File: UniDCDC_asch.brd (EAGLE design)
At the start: 35.2 x 35.9 mm, 13 parts

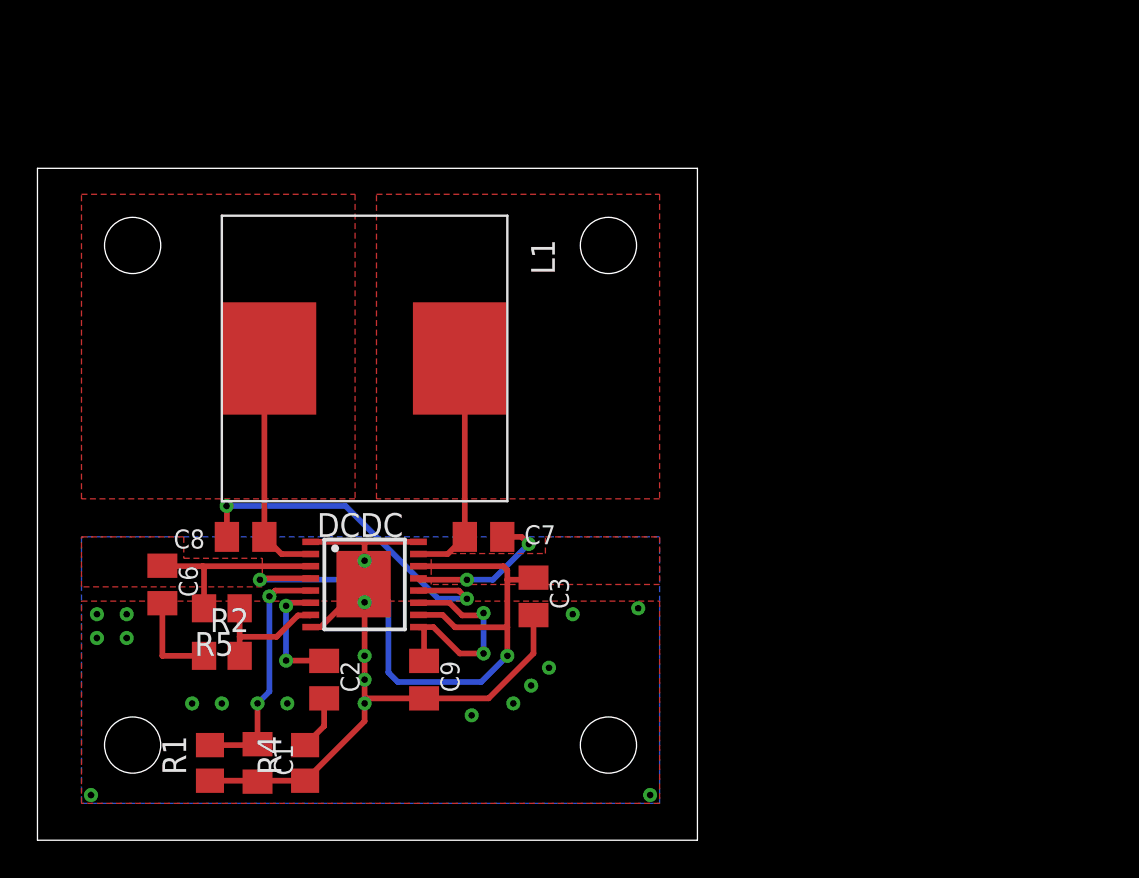
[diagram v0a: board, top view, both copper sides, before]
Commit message: Manufacturing version
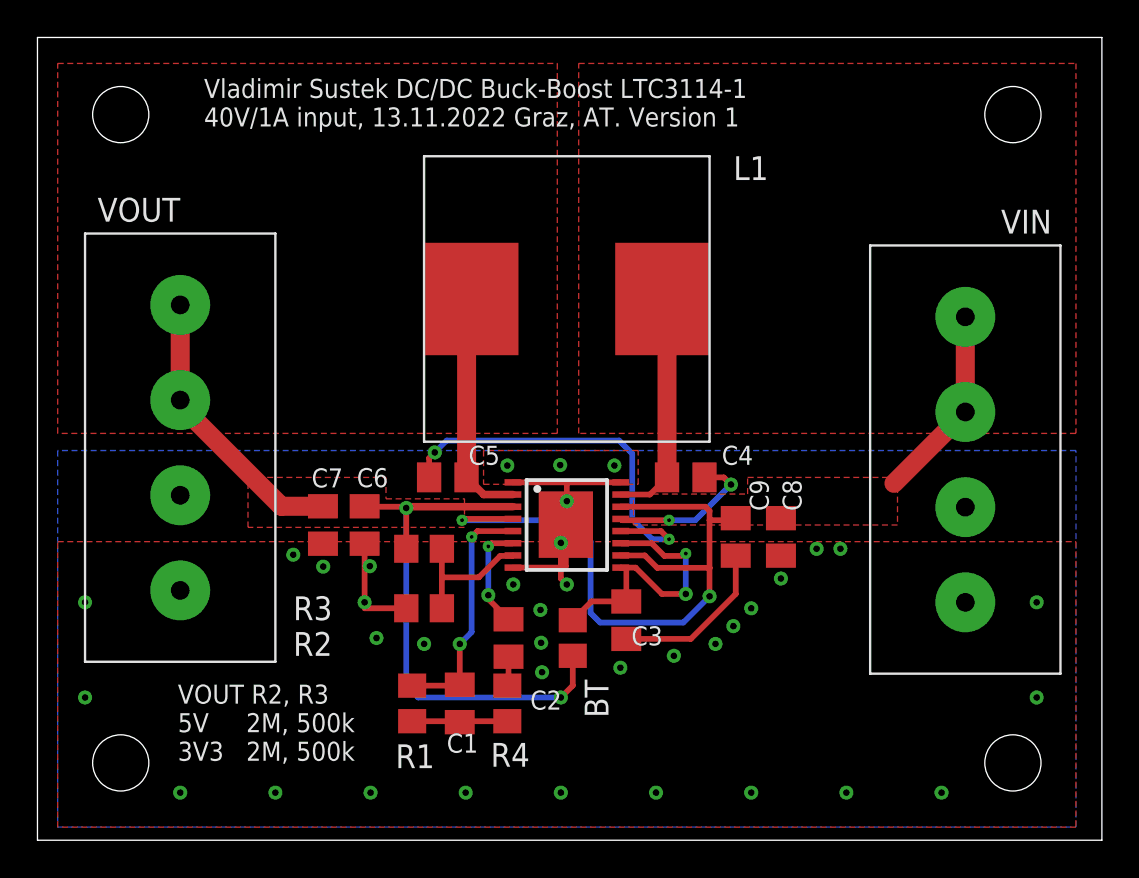
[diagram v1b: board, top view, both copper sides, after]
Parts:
- removed R5: (no value), rcl:R0805
- added BT: DNI, rcl:R0805
- added C4, C5: 68nF, rcl:C0805K
- added R3: 2M, rcl:R0805
- added VIN, VOUT: SCREW_TERMINAL, uni_dcdc:SCREW_TERMINAL
- C1: value (none) -> 33nF
- C2: value (none) -> 4.7nF
- C3: value (none) -> 4.7uF
- C6, C7: value (none) -> 30uF
- C8, C9: value (none) -> 10uF
- L1: value MSS1278 -> 6.8-15uH
- R1: value (none) -> 20k
- R2: value (none) -> 500k
- R4: value (none) -> 27.4k
- moved C8 28.6 mm to (39.7, 16.2), turned to 270 degrees
- moved C9 18.3 mm to (37.3, 16.2)
- moved DCDC 11.3 mm to (28.3, 16.8)
- moved R1 11.3 mm to (20.0, 7.30)
- moved C1 11.3 mm to (22.5, 7.30)
- moved L1 11.3 mm to (28.3, 28.9)
- moved R4 11.3 mm to (25.1, 7.30)
- moved C6 11.3 mm to (17.5, 16.8)
- moved R2 11.1 mm to (20.6, 12.4)
- moved C2 10.1 mm to (25.1, 10.8)
- moved C7 8.60 mm to (15.2, 16.8), turned to 270 degrees
- moved C3 5.11 mm to (31.4, 11.7)
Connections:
- net BST1: now also C4.2; no longer C7.2
- net BST2: now also C5.2; no longer C8.2
- net FB: now also R3.1; no longer R5.1
- net GND: now also C7.2, C8.2, VIN.P$1, VIN.P$2, VOUT.P$1, VOUT.P$2
- net LDO: now also BT.1, C3.1; no longer C9.1
- net N$11: now also C4.1; no longer C7.1
- net N$12: now also C5.1; no longer C8.1
- net VIN: now also C8.1, C9.1, VIN.P$3, VIN.P$4; no longer C3.1
- net VOUT: now also BT.2, C7.1, R3.2, VOUT.P$3, VOUT.P$4; no longer R5.2
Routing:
- net VOUT: track 10.2 -> 45.9 mm, vias 0 -> 2
- net VIN: track 36.9 -> 47.4 mm
- net GND: track 45.9 -> 36.2 mm, vias 20 -> 24
- net LDO: track 12.2 -> 15.5 mm
- net BST2: track 19.3 -> 21.2 mm
- net N$6: track 2.92 -> 1.57 mm
- net FB: track 6.82 -> 7.45 mm
- net VC: track 6.35 -> 5.72 mm
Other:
- board size 35.2 x 35.9 mm -> 56.8 x 42.9 mm
- board text added: "VOUT R2, R3 5V 2M, 500k 3V3 2M, 500k"
- board text added: "Vladimir Sustek DC/DC Buck-Boost LTC3114-1 40V/1A input, 13.11.2022 Graz, AT. Version 1"
